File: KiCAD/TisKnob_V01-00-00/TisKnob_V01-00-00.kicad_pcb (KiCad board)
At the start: 2 copper layers, 94 x 31.4 mm, 119 parts, among them J1 86091325113755E1LF, J2 Conn_02x03_Odd_Even, K1 TLP3451, K2 TLP3451, K3 TLP3451, K4 TLP3451, K5 TLP3451, K6 TLP3451, K7 TLP3451, Q1 Q_NMOS, Q2 BSS192PH6327FTSA1, Q3 BSS123, Q4 BSS192PH6327FTSA1, U1 OPA994IDCKR, U10 OPA994IDCKR, U11 STM32G474CETx, U12 OPA994IDCKR, U13 OPA994IDCKR, U2 OPA994IDCKR, U5 LT6654BHS6-3.3#WTRMPBF, U6 TPS62932, U7 TS12A12511DCN, U8 TLV1841DCKR, U9 INA193

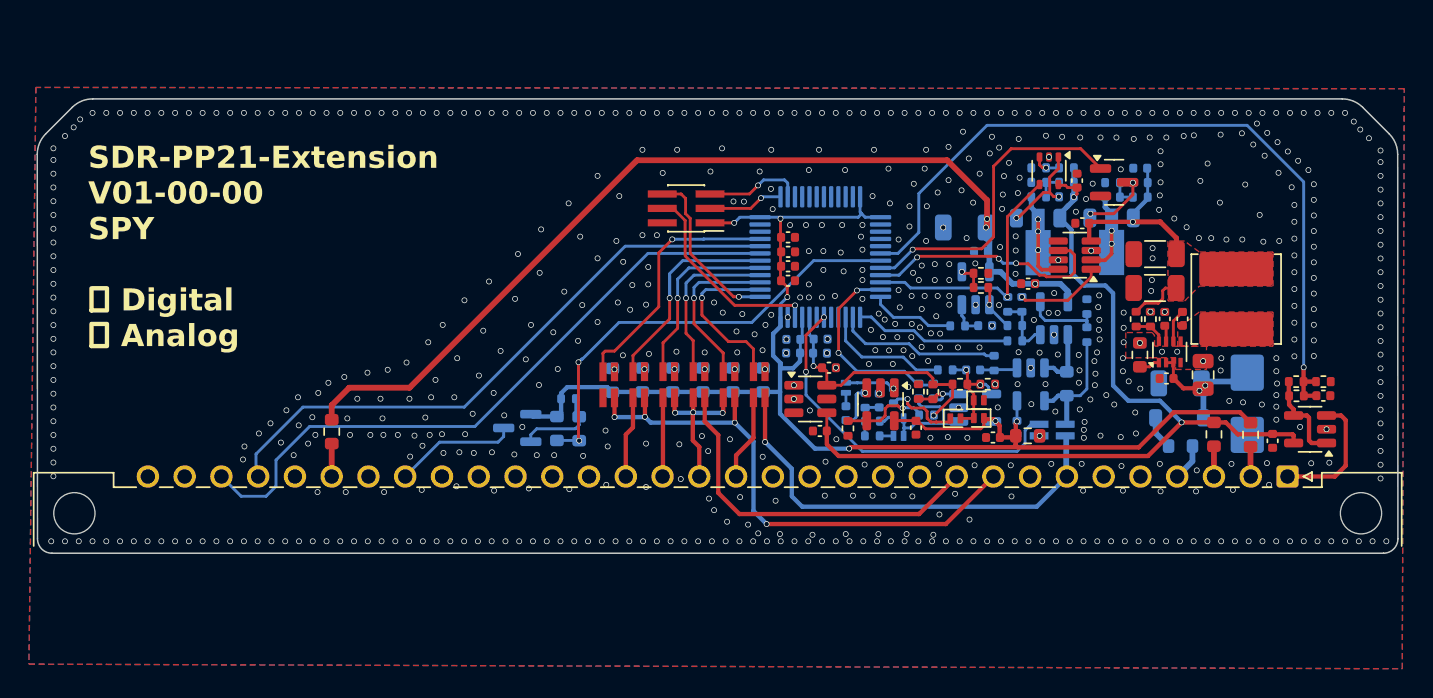
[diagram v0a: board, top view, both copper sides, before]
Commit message: KiCAD
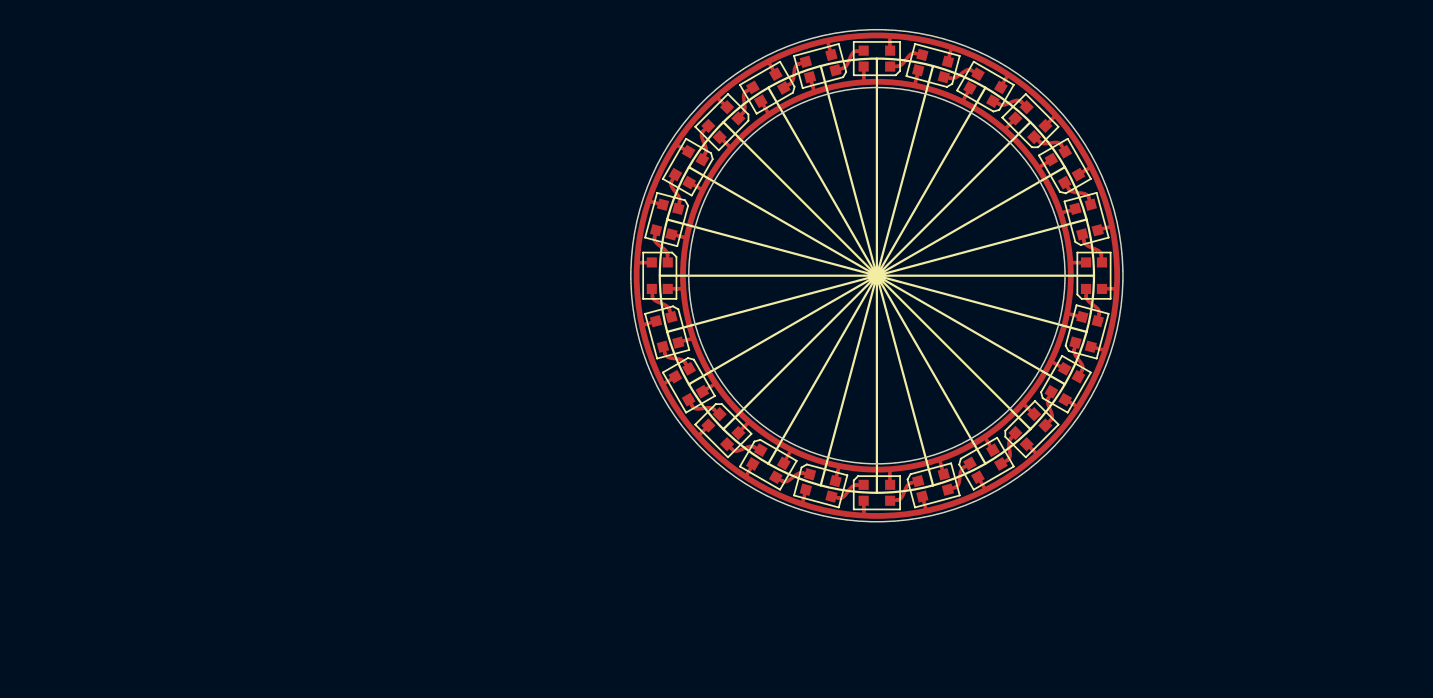
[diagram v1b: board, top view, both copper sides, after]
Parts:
- removed C10, C12, C14, C18, C20, C23, C24, C25, C26, C3, C32, C33, C35, C36, C37, C4, C5, C9: 100n, Capacitor_SMD:C_0402_1005Metric
- removed C13, C8: 1u, Capacitor_SMD:C_0402_1005Metric
- removed C15, C6: 4u7, Capacitor_SMD:C_0402_1005Metric
- removed C17: 10u, Capacitor_SMD:C_0805_2012Metric
- removed C19: 33nF, Capacitor_SMD:C_0402_1005Metric
- removed C21, C22: 22u, Capacitor_SMD:C_1206_3216Metric
- removed C27: 1n, Capacitor_SMD:C_0402_1005Metric
- removed C29, C30, C7: 10n, Capacitor_SMD:C_0402_1005Metric
- removed C50, C51: 10u, Capacitor_SMD:C_1206_3216Metric
- removed J1: 86091325113755E1LF, SDR_Connector:DIN41612_B_1x32_Male_Horizontal_THT
- removed J2: Conn_02x03_Odd_Even, Connector_PinHeader_1.00mm:PinHeader_2x03_P1.00mm_Vertical_SMD
- removed K1, K2, K3, K4, K5, K6, K7: TLP3451, SDR_IC:VSON-4
- removed L1: 15uH, SDR_INDCUTOR:L_Bourns_SRN6045TA
- removed Q1: Q_NMOS, Package_TO_SOT_SMD:SOT-23
- removed Q2, Q4: BSS192PH6327FTSA1, Package_TO_SOT_SMD:SOT-89-3
- removed Q3: BSS123, Package_TO_SOT_SMD:SOT-23
- removed R1, R18, R19, R2, R3, R4, R46: 0, Resistor_SMD:R_0603_1608Metric
- removed R10, R5, R6, R60, R7, R8, R9: 200, Resistor_SMD:R_0603_1608Metric
- removed R11: R, Resistor_SMD:R_0402_1005Metric
- removed R20: 84k5, Resistor_SMD:R_0402_1005Metric
- removed R21, R32, R35, R36, R37, R40, R41, R43, R44, R45, R48, R49, R50, R52, R54, R55, R56, R58, R61: 10k, Resistor_SMD:R_0402_1005Metric
- removed R22, R26, R39: 1k, Resistor_SMD:R_0402_1005Metric
- removed R23, R27, R29, R30: 2k, Resistor_SMD:R_0402_1005Metric
- removed R24: 4.02k, Resistor_SMD:R_0402_1005Metric
- removed R25: 200k, Resistor_SMD:R_0402_1005Metric
- removed R28: 8.06k, Resistor_SMD:R_0402_1005Metric
- removed R31: 3k, Resistor_SMD:R_0402_1005Metric
- removed R33, R34: x, Resistor_SMD:R_0402_1005Metric
- removed R38: 2k4, Resistor_SMD:R_0402_1005Metric
- removed R42: 100k, Resistor_SMD:R_0402_1005Metric
- removed R51, R57: 20k, Resistor_SMD:R_0402_1005Metric
- removed R53: 100, Resistor_SMD:R_0402_1005Metric
- removed R59: 1, Resistor_SMD:R_0603_1608Metric
- removed U1, U10, U12, U13, U2: OPA994IDCKR, Package_TO_SOT_SMD:SOT-23-5
- removed U11: STM32G474CETx, Package_QFP:LQFP-48_7x7mm_P0.5mm
- removed U5: LT6654BHS6-3.3#WTRMPBF, Package_TO_SOT_SMD:SOT-23-6
- removed U6: TPS62932, Package_TO_SOT_SMD:SOT-583-8
- removed U7: TS12A12511DCN, Package_TO_SOT_SMD:SOT-23-8
- removed U8: TLV1841DCKR, Package_TO_SOT_SMD:SOT-353_SC-70-5
- removed U9: INA193, Package_TO_SOT_SMD:SOT-23-5
- added D10: WS2812B-2020, TouchKnob:LED_WS2812B-2020_PLCC4_2.0x2.0mm, F.Cu at (260.6, 110.6)
- added D11: WS2812B-2020, TouchKnob:LED_WS2812B-2020_PLCC4_2.0x2.0mm, F.Cu at (257.5, 113.0)
- added D12: WS2812B-2020, TouchKnob:LED_WS2812B-2020_PLCC4_2.0x2.0mm, F.Cu at (253.9, 114.5)
- added D13: WS2812B-2020, TouchKnob:LED_WS2812B-2020_PLCC4_2.0x2.0mm, F.Cu at (250.0, 115.0)
- added D14: WS2812B-2020, TouchKnob:LED_WS2812B-2020_PLCC4_2.0x2.0mm, F.Cu at (246.1, 114.5)
- added D15: WS2812B-2020, TouchKnob:LED_WS2812B-2020_PLCC4_2.0x2.0mm, F.Cu at (242.5, 113.0)
- added D16: WS2812B-2020, TouchKnob:LED_WS2812B-2020_PLCC4_2.0x2.0mm, F.Cu at (239.4, 110.6)
- added D17: WS2812B-2020, TouchKnob:LED_WS2812B-2020_PLCC4_2.0x2.0mm, F.Cu at (237.0, 107.5)
- added D18: WS2812B-2020, TouchKnob:LED_WS2812B-2020_PLCC4_2.0x2.0mm, F.Cu at (235.5, 103.9)
- added D19: WS2812B-2020, TouchKnob:LED_WS2812B-2020_PLCC4_2.0x2.0mm, F.Cu at (235.0, 100.0)
- added D20: WS2812B-2020, TouchKnob:LED_WS2812B-2020_PLCC4_2.0x2.0mm, F.Cu at (235.5, 96.1)
- added D21: WS2812B-2020, TouchKnob:LED_WS2812B-2020_PLCC4_2.0x2.0mm, F.Cu at (237.0, 92.5)
- added D22: WS2812B-2020, TouchKnob:LED_WS2812B-2020_PLCC4_2.0x2.0mm, F.Cu at (239.4, 89.4)
- added D23: WS2812B-2020, TouchKnob:LED_WS2812B-2020_PLCC4_2.0x2.0mm, F.Cu at (242.5, 87.0)
- added D24: WS2812B-2020, TouchKnob:LED_WS2812B-2020_PLCC4_2.0x2.0mm, F.Cu at (246.1, 85.5)
- added D9: WS2812B-2020, TouchKnob:LED_WS2812B-2020_PLCC4_2.0x2.0mm, F.Cu at (263.0, 107.5)
- D1: value SM6T27A -> WS2812B-2020; footprint Diode_SMD:D_SMB -> TouchKnob:LED_WS2812B-2020_PLCC4_2.0x2.0mm; moved to F.Cu
- D2: value SD103AW-HE3_A-08 -> WS2812B-2020; footprint Diode_SMD:D_SOD-123 -> TouchKnob:LED_WS2812B-2020_PLCC4_2.0x2.0mm; moved to F.Cu
- D3, D4, D7: value BAT32ALS-QYL -> WS2812B-2020; footprint Diode_SMD:D_SOD-882 -> TouchKnob:LED_WS2812B-2020_PLCC4_2.0x2.0mm
- D5, D6, D8: value BAT32ALS-QYL -> WS2812B-2020; footprint Diode_SMD:D_SOD-882 -> TouchKnob:LED_WS2812B-2020_PLCC4_2.0x2.0mm; moved to F.Cu
- moved D1 35.0 mm to (250.0, 85.0), turned to 180 degrees
- moved D2 29.7 mm to (253.9, 85.5), turned to 165 degrees
- moved D3 22.8 mm to (257.5, 87.0), turned to 150 degrees
- moved D5 20.8 mm to (263.0, 92.5), turned to 120 degrees
- moved D6 19.8 mm to (264.5, 96.1), turned to 105 degrees
- moved D4 19.5 mm to (260.6, 89.4), turned to 135 degrees
- moved D8 17.1 mm to (264.5, 103.9), turned to 75 degrees
- moved D7 13.7 mm to (265.0, 100.0), turned to 90 degrees
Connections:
- D1 pad 1: +24V -> Net-(D1-DOUT)
- D1 pad 2: GND -> Net-(D1-VSS)
- D2 pad 1: +24V -> Net-(D2-DOUT)
- D2 pad 2: Net-(D2-A) -> Net-(D1-VSS)
- D3 pad 1: +3V3 -> Net-(D3-DOUT)
- D3 pad 2: Net-(D3-A) -> Net-(D1-VSS)
- D4 pad 1: Net-(D3-A) -> Net-(D4-DOUT)
- D4 pad 2: GND -> Net-(D1-VSS)
- D5 pad 1: Net-(D5-K) -> Net-(D5-DOUT)
- D5 pad 2: /SDR_OWI_Rx/LEVEL -> Net-(D1-VSS)
- D6 pad 1: /SDR_OWI_Rx/LEVEL -> Net-(D6-DOUT)
- D6 pad 2: Net-(D6-A) -> Net-(D1-VSS)
- D7 pad 1: R_LEVEL -> Net-(D7-DOUT)
- D7 pad 2: Net-(D3-A) -> Net-(D1-VSS)
- D8 pad 2: Net-(D8-A) -> Net-(D1-VSS)
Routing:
- net +3V3: track 100.4 -> 0.00 mm, vias 6 -> 0
- net +12V: track 66.2 -> 0.00 mm, vias 3 -> 0
- net +5V: track 62.5 -> 0.00 mm, vias 2 -> 0
- net V_ADC: track 52.6 -> 0.00 mm, vias 1 -> 0
- net SDR_Tx: track 45.8 -> 0.00 mm
- net SDR_Rx: track 42.4 -> 0.00 mm
- net SIG_V-: track 37.9 -> 0.00 mm, vias 4 -> 0
- net NRST: track 30.8 -> 0.00 mm, vias 2 -> 0
- net SIG_V+: track 30.6 -> 0.00 mm, vias 1 -> 0
- net S_SIG: track 25.1 -> 0.00 mm
- net Con_OWI: track 24.9 -> 0.00 mm, vias 2 -> 0
- net OWI_ACTIV: track 22.1 -> 0.00 mm, vias 1 -> 0
- net +3V3_REF: track 18.1 -> 0.00 mm, vias 2 -> 0
- net OWI_Tx: track 17.9 -> 0.00 mm, vias 1 -> 0
- net Con_GND: track 17.6 -> 0.00 mm, vias 1 -> 0
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- removed copper zone on F.Cu, net +7.5V
- removed copper zone on B.Cu, net GND
- removed copper zone on F.Cu, net GND
- removed copper zone on F.Cu, net Net-(U6-SW)
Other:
- board size 94 x 31.4 mm -> 34 x 34 mm
- board text removed: "SDR-PP21-Extension V01-00-00 SPY ⬜ Digital ⬜ Analog"
